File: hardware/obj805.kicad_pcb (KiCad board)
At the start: 2 copper layers, 65 x 56.5 mm, 8 parts, among them J0 Conn_with_rapi, P0 Jack-DC, U1 L293D

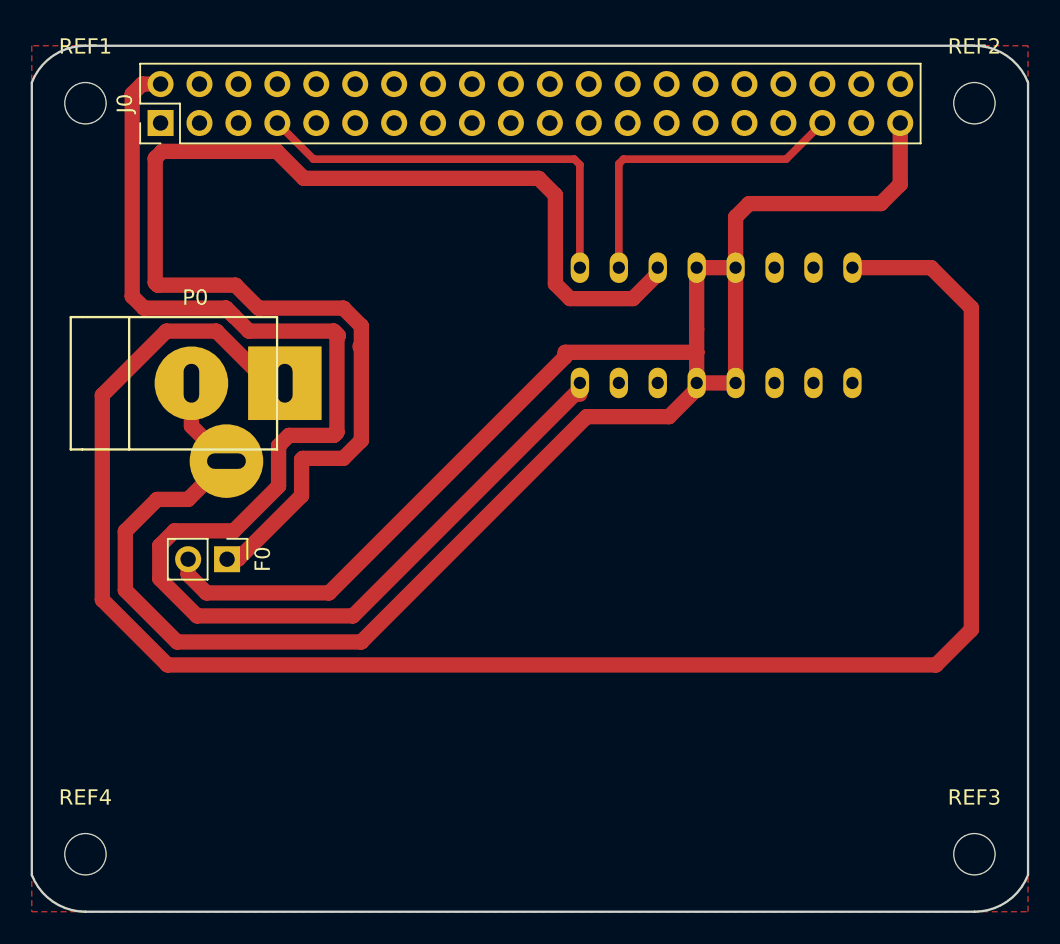
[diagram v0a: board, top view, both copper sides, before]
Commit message: update
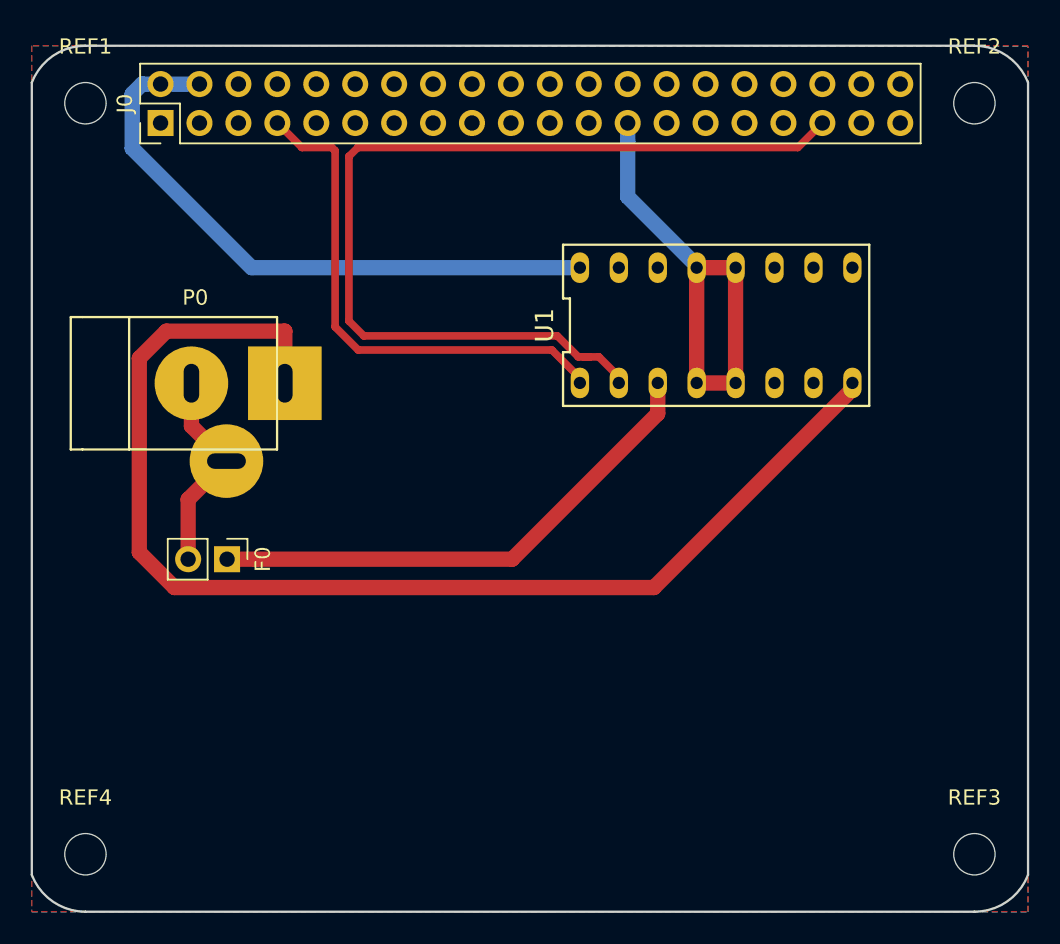
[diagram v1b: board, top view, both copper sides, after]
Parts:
- U1: moved to F.Cu
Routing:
- net Net-(F0-Pad2): track 144.7 -> 44.9 mm
- net Net-(F0-Pad1): track 85.2 -> 34.0 mm
- net Net-(J0-Pad2): track 91.2 -> 40.6 mm
- net Net-(J0-Pad35): track 21.2 -> 62.5 mm
- net Net-(P0-Pad1): track 117.7 -> 79.5 mm
- net Net-(J0-Pad7): track 27.6 -> 33.7 mm
- added copper zone on B.Cu, net Net-(F0-Pad2)
